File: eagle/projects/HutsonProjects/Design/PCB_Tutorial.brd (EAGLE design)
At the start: 160 x 100 mm, 15 parts, among them J1 POWER_JACKPTH_BREAD, J3 AVR_SPI_PROG_3X2PTH, J4 6_PIN_SERIAL_CABLEPTH, U1 328P

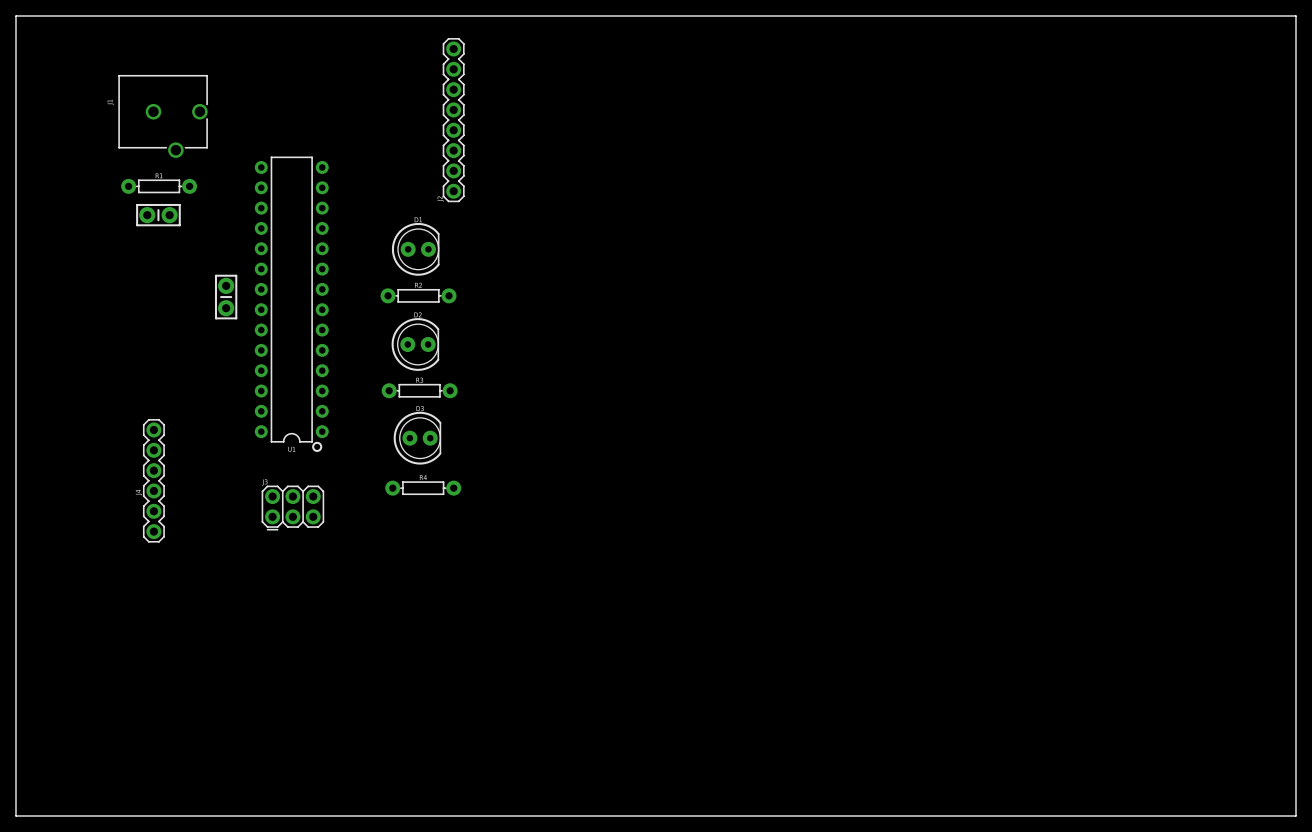
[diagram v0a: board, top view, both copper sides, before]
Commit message: Dimensions
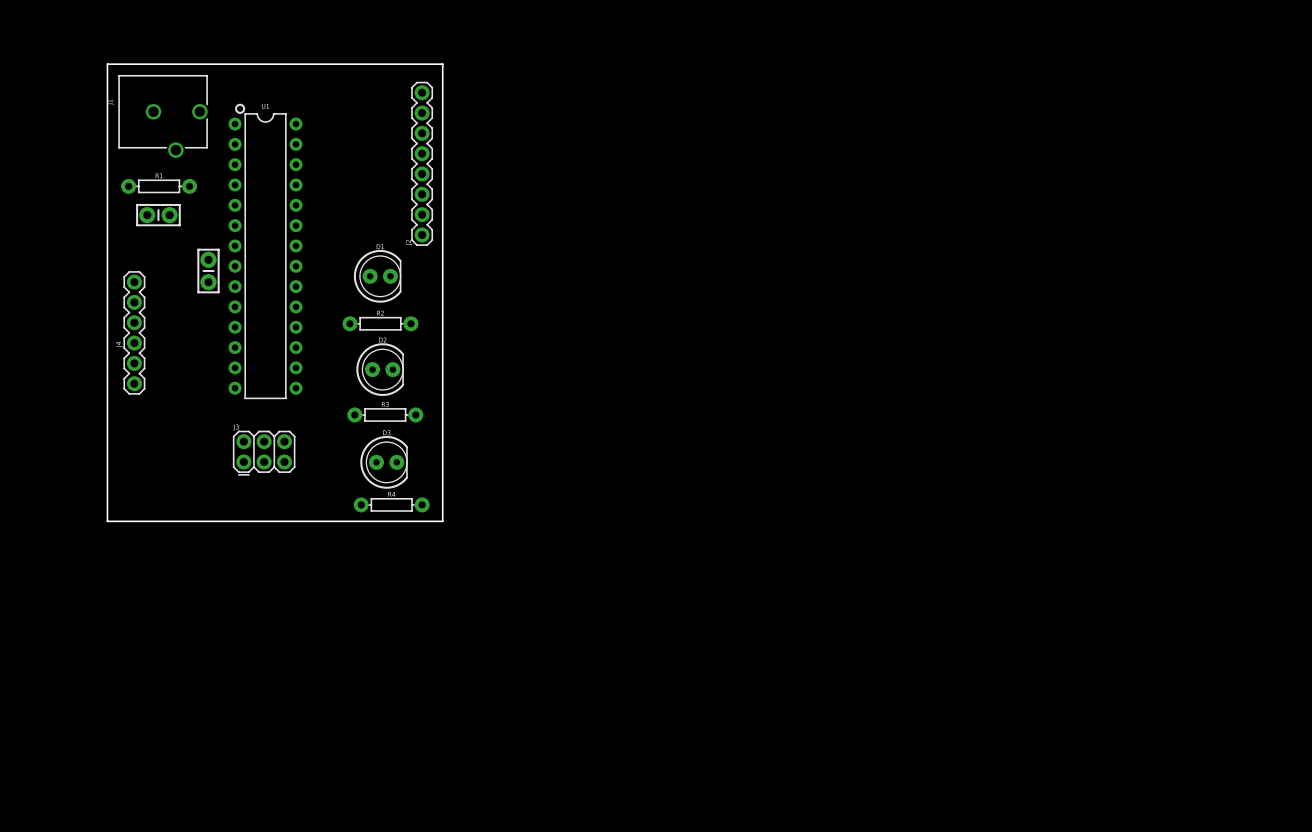
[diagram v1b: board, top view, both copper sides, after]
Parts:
- moved J4 18.6 mm to (14.8, 54.0)
- moved J3 7.75 mm to (28.5, 44.3)
- moved J2 6.74 mm to (50.8, 72.6)
- moved U1 6.34 mm to (31.2, 70.0), turned to 270 degrees
- moved R2 5.90 mm to (45.6, 61.5)
- moved D1 5.83 mm to (45.5, 67.5)
- moved D2 5.41 mm to (45.8, 55.8)
- moved R3 5.25 mm to (46.2, 50.1)
- moved D3 5.16 mm to (46.3, 44.2)
- moved R4 4.47 mm to (47.0, 38.9)
- moved C2 3.93 mm to (24.1, 68.1)
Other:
- board size 160 x 100 mm -> 41.9 x 57.2 mm
